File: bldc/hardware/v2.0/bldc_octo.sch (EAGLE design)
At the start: 11 parts, among them J1 PWR_2_XT30PW-M, J2 LINEAR_3_MOLEX_5023520300, J3 LINEAR_3_AMASS_MR30PW-M, U1 MA702, U2 STM32H723VGT6, U3 DRV8323RS, U4 MCP2542FD, X1 CRYSTAL_NX2016SA-24MHZ-EXS00A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

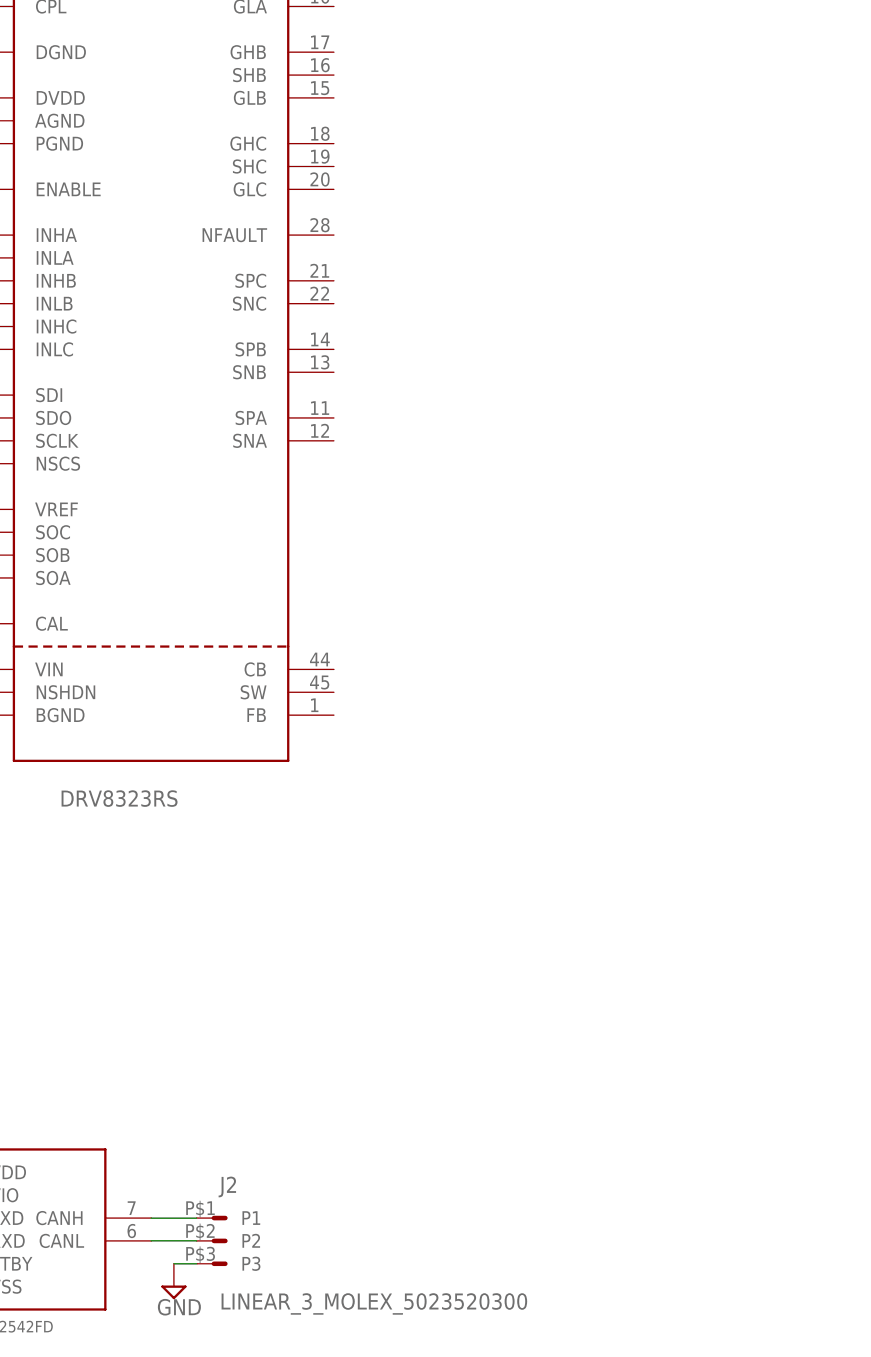
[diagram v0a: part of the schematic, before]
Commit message: Going to start can
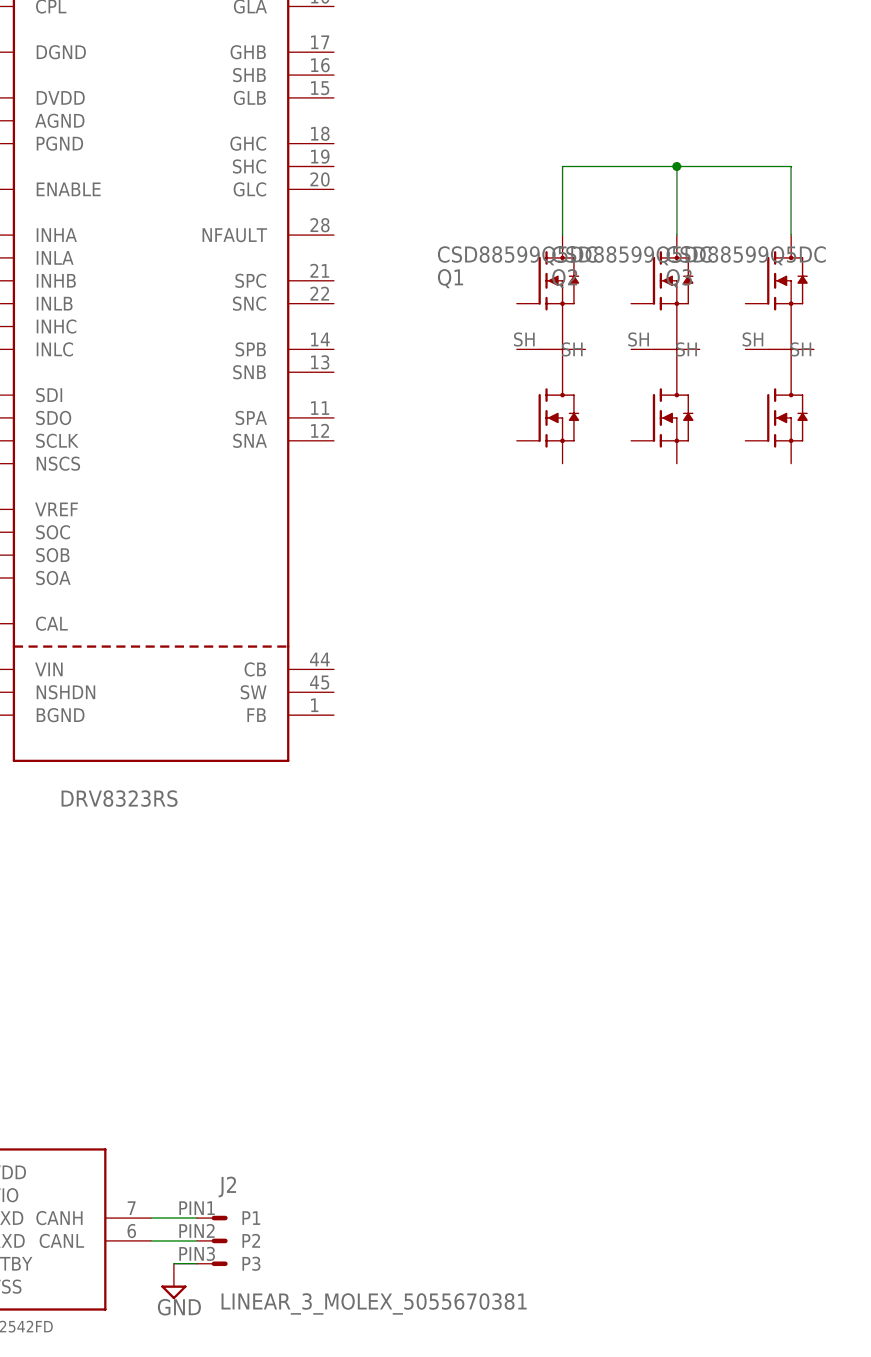
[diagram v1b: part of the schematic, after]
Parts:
- added Q1, Q2, Q3: CSD88599Q5DC, _T_transistors:CSD88599Q5DC
- J2: value LINEAR_3_MOLEX_5023520300 -> LINEAR_3_MOLEX_5055670381; device _T_conn:LINEAR_3_MOLEX_5023520300 -> _T_conn:LINEAR_3_MOLEX_5055670381
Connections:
- new net N$5: Q1.V_IN, Q2.V_IN, Q3.V_IN
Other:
- moved on the sheet: J2
